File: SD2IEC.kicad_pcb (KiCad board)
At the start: 2 copper layers, 64 x 50 mm, 49 parts, among them J1 AVR-ISP-6, J2 5VDC IN, J3 SD_Card, J4 IEC (DIN6), J5 IEC (DIN6), J6 SERIAL, J7 I2C, J8 IEC_ALT1, J9 IEC_ALT2, Q1 AO3400A, Q2 AO3400A, Q3 AO3400A, SW1 IEC_SEL, SW2 PREV, SW3 NEXT, SW4 RESET, U1 ATmega1284P-20AU, U2 MIC5504-3.3YM5, Y1 8MHz

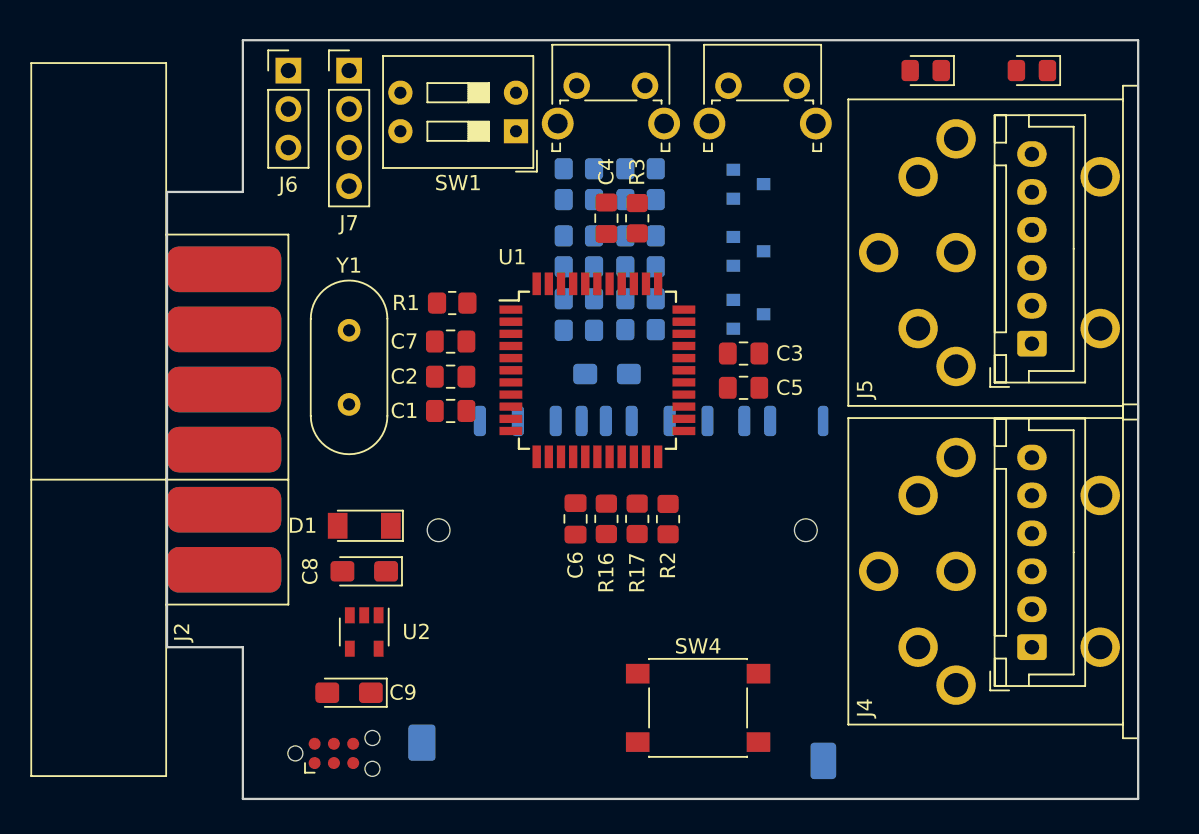
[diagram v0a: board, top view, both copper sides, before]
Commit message: Begin routing
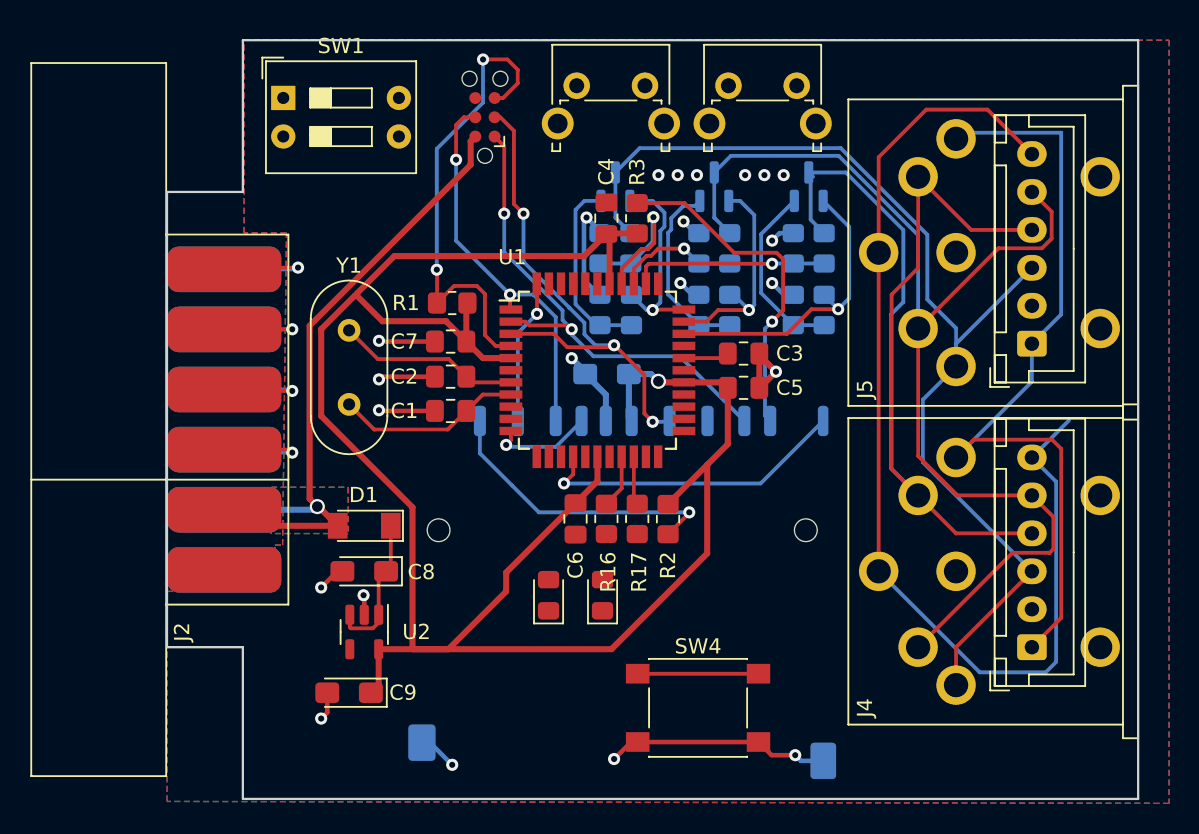
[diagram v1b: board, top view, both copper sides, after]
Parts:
- removed J6: SERIAL, Connector_PinHeader_2.54mm:PinHeader_1x03_P2.54mm_Vertical
- removed J7: I2C, Connector_PinHeader_2.54mm:PinHeader_1x04_P2.54mm_Vertical
- moved D3 47.0 mm to (109.0, 115.2), turned to 90 degrees
- moved J1 43.1 mm to (104.8, 83.7), turned to 90 degrees
- moved D2 40.6 mm to (112.5, 115.2), turned to 90 degrees
- moved R4 17.7 mm to (127.1, 96.4), turned to 90 degrees
- moved R5 16.9 mm to (125.1, 96.4), turned to 90 degrees
- moved SW1 15.5 mm to (91.5, 82.5), turned to 0 degrees
- moved R6 12.5 mm to (127.1, 92.4), turned to -90 degrees
- moved Q3 12.1 mm to (113.4, 88.3), turned to 90 degrees
- moved R7 11.4 mm to (125.1, 92.4), turned to 90 degrees
- moved R8 10.3 mm to (120.9, 96.4), turned to 90 degrees
- moved R9 9.29 mm to (118.9, 96.4), turned to 90 degrees
- moved R10 6.00 mm to (120.9, 92.4), turned to -90 degrees
- moved R14 5.40 mm to (114.4, 92.4), turned to -90 degrees
- moved Q2 4.82 mm to (119.9, 88.3), turned to 90 degrees
- moved R15 4.27 mm to (112.4, 92.4), turned to 90 degrees
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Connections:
- J2 pad 3: (no net) -> unconnected-(J2-Pad3)
- J2 pad 4: (no net) -> unconnected-(J2-Pad4)
- J2 pad 5: (no net) -> unconnected-(J2-Pad5)
- J2 pad 6: (no net) -> unconnected-(J2-Pad6)
- U1 pad 10: /TXD -> unconnected-(U1-Pad10)
- U1 pad 23: /SCL -> unconnected-(U1-Pad23)
- U1 pad 24: /SDA -> unconnected-(U1-Pad24)
- U1 pad 25: /INTRQ -> unconnected-(U1-Pad25)
- U1 pad 9: /RXD -> unconnected-(U1-Pad9)
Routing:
- net +3.3V: track 0.00 -> 136.5 mm, vias 0 -> 1
- net /IEC_DATA: track 0.00 -> 74.2 mm
- net /IEC_ATN: track 0.00 -> 73.0 mm
- net /~{IEC_RESET}: track 0.00 -> 72.2 mm
- net /IEC_CLK: track 0.00 -> 71.1 mm
- net GND: track 0.00 -> 57.5 mm, vias 0 -> 22
- net /~{IEC_SQR}: track 0.00 -> 52.9 mm
- net +5V: track 0.00 -> 45.1 mm, vias 0 -> 1
- net Net-(J1-Pad5): track 0.00 -> 39.2 mm, vias 0 -> 2
- net /SCK: track 0.00 -> 33.7 mm, vias 0 -> 3
- net /MISO: track 0.00 -> 33.1 mm, vias 0 -> 2
- net /MOSI: track 0.00 -> 25.6 mm, vias 0 -> 2
- net Net-(J3-Pad8): track 0.00 -> 22.4 mm, vias 0 -> 1
- net /~{WRITE_PROTECT}: track 0.00 -> 20.8 mm, vias 0 -> 1
- net /IEC_CLK/WRITE: track 0.00 -> 20.3 mm, vias 0 -> 1
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- added copper zone on B.Cu, net +5V
- added copper zone on F.Cu, net +5V
- added copper zone on B.Cu, net GND
- added copper zone on F.Cu, net GND
